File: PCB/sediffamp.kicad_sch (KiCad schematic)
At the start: 19 parts, among them U13 OPA1622

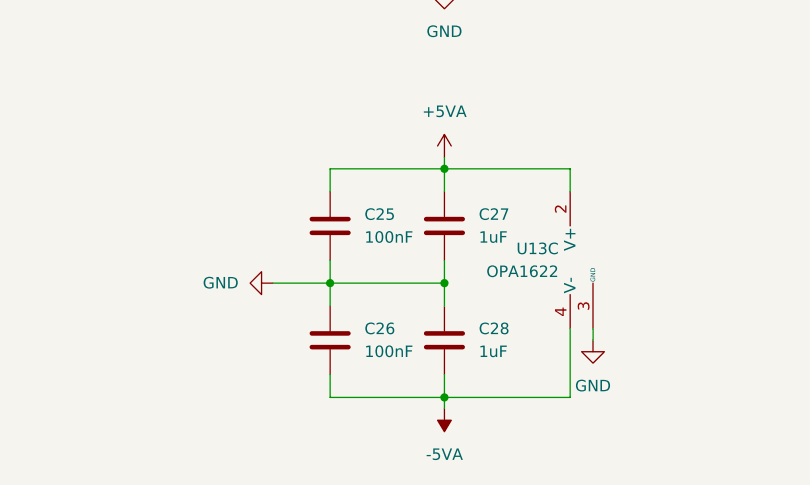
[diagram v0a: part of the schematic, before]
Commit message: Redone placement and layout of OPA1622. Still finishing touches
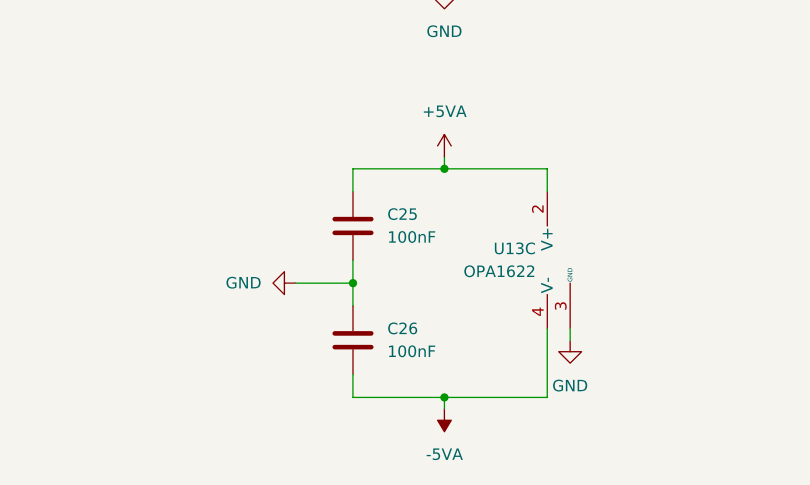
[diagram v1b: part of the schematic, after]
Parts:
- removed C27, C28: 1uF, Capacitor_SMD:C_0603_1608Metric_Pad1.08x0.95mm_HandSolder, symbol Device:C
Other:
- moved on the sheet: C25, C26, U13C
